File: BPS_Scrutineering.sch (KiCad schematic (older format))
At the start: 26 parts, among them J1 Conn_01x01_Female, J10 Conn_01x01_Female, J11 Conn_01x01_Female, J12 Conn_01x01_Female, J13 Conn_01x01_Female, J14 Conn_01x01_Female, J2 Conn_01x01_Female, J3 Conn_01x01_Female, J4 Conn_01x01_Female, J5 Conn_01x01_Female, J6 Conn_01x01_Female, J7 Conn_01x01_Female, J8 Conn_01x01_Female, J9 Conn_01x01_Female, SW1 SW_DIP_x07, SW2 SW_DIP_x07

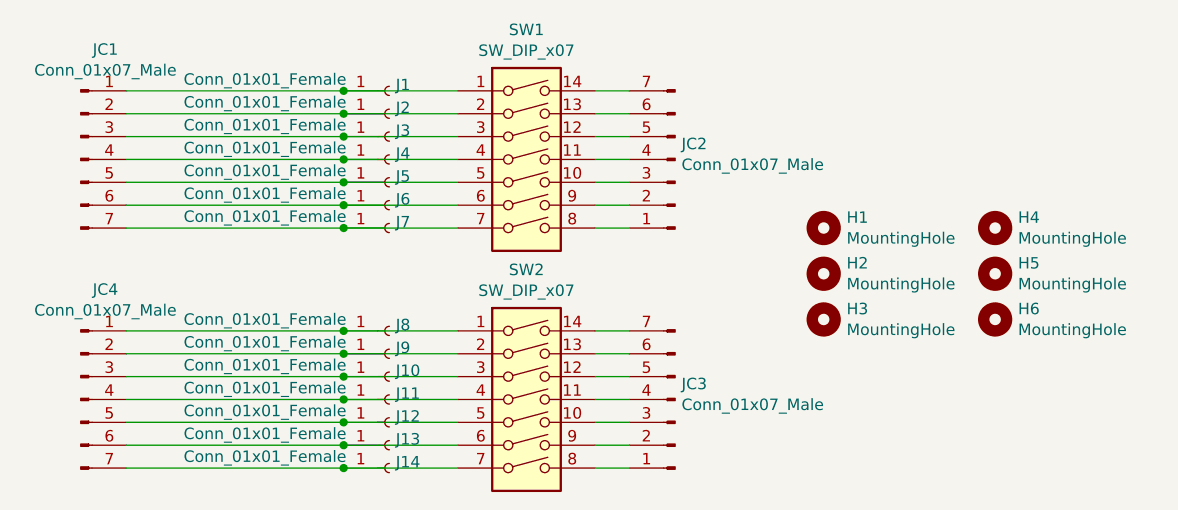
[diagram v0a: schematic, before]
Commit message: Finished PCB
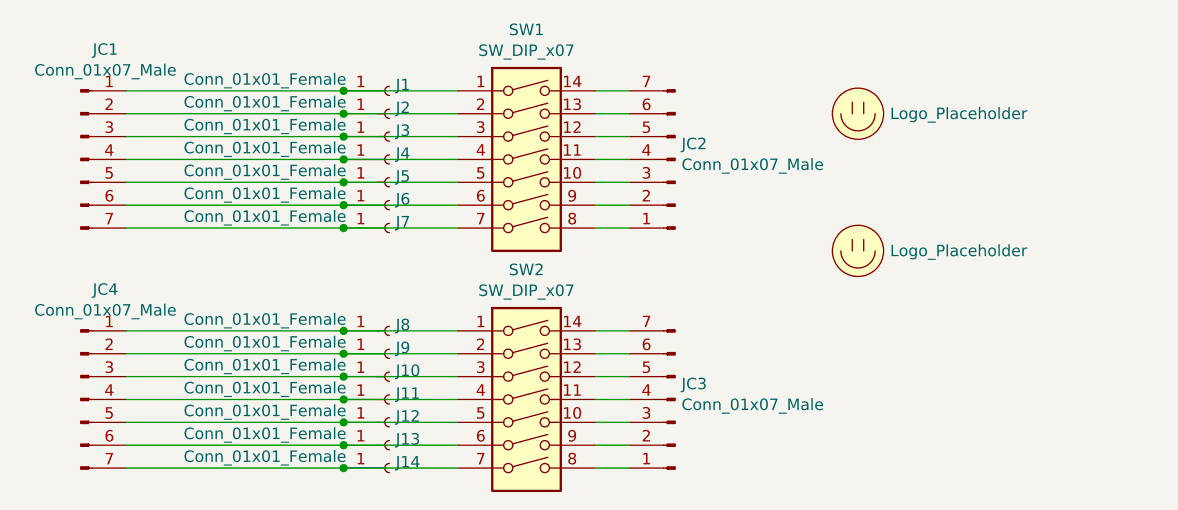
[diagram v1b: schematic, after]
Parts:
- removed H1, H2, H3, H4, H5, H6: MountingHole, MountingHole:MountingHole_3mm, symbol Mechanical:MountingHole
- added LOGO1: Logo_Placeholder, UTSVT_Special:UTSVT_Logo_Symbol, symbol utsvt-misc:Logo_Placeholder
- added LOGO2: Logo_Placeholder, UTSVT_Special:Hallock_Image, symbol utsvt-misc:Logo_Placeholder
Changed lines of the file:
@@
-$EndComp
-$Comp
-L Mechanical:MountingHole H1
-U 1 1 5F9473C1
-P 4650 2000
-F 0 "H1" H 4750 2046 50  0000 L CNN
-F 1 "MountingHole" H 4750 1955 50  0000 L CNN
-F 2 "MountingHole:MountingHole_3mm" H 4650 2000 50  0001 C CNN
-F 3 "~" H 4650 2000 50  0001 C CNN
-	1    4650 2000
-	1    0    0    -1
 $EndComp
 $Comp
@@
 $EndComp
 $Comp
-L Mechanical:MountingHole H2
-U 1 1 5FAEC2DE
-P 4650 2200
-F 0 "H2" H 4750 2246 50  0000 L CNN
-F 1 "MountingHole" H 4750 2155 50  0000 L CNN
-F 2 "MountingHole:MountingHole_3mm" H 4650 2200 50  0001 C CNN
-F 3 "~" H 4650 2200 50  0001 C CNN
-	1    4650 2200
-	1    0    0    -1
-$EndComp
-$Comp
-L Mechanical:MountingHole H3
-U 1 1 5FAF0045
-P 4650 2400
-F 0 "H3" H 4750 2446 50  0000 L CNN
-F 1 "MountingHole" H 4750 2355 50  0000 L CNN
-F 2 "MountingHole:MountingHole_3mm" H 4650 2400 50  0001 C CNN
-F 3 "~" H 4650 2400 50  0001 C CNN
-	1    4650 2400
-	1    0    0    -1
-$EndComp
-$Comp
-L Mechanical:MountingHole H4
-U 1 1 5FAF40EC
-P 5400 2000
-F 0 "H4" H 5500 2046 50  0000 L CNN
-F 1 "MountingHole" H 5500 1955 50  0000 L CNN
-F 2 "MountingHole:MountingHole_3mm" H 5400 2000 50  0001 C CNN
-F 3 "~" H 5400 2000 50  0001 C CNN
-	1    5400 2000
-	1    0    0    -1
-$EndComp
-$Comp
-L Mechanical:MountingHole H5
-U 1 1 5FAF7F09
-P 5400 2200
-F 0 "H5" H 5500 2246 50  0000 L CNN
-F 1 "MountingHole" H 5500 2155 50  0000 L CNN
-F 2 "MountingHole:MountingHole_3mm" H 5400 2200 50  0001 C CNN
-F 3 "~" H 5400 2200 50  0001 C CNN
-	1    5400 2200
-	1    0    0    -1
-$EndComp
-$Comp
-L Mechanical:MountingHole H6
-U 1 1 5FAFBD75
-P 5400 2400
-F 0 "H6" H 5500 2446 50  0000 L CNN
-F 1 "MountingHole" H 5500 2355 50  0000 L CNN
-F 2 "MountingHole:MountingHole_3mm" H 5400 2400 50  0001 C CNN
-F 3 "~" H 5400 2400 50  0001 C CNN
-	1    5400 2400
-	1    0    0    -1
-$EndComp
-$Comp
 L Switch:SW_DIP_x07 SW1
 U 1 1 5FADB5F5
@@
 Wire Wire Line
 	3800 3050 3650 3050
+$Comp
+L utsvt-misc:Logo_Placeholder LOGO1
+U 1 1 5FB02C91
+P 4800 2100
+F 0 "LOGO1" H 4800 2250 50  0001 C CNN
+F 1 "Logo_Placeholder" H 4940 2100 50  0000 L CNN
+F 2 "UTSVT_Special:UTSVT_Logo_Symbol" H 4800 2175 50  0001 C CNN
+F 3 "" H 4800 2175 50  0001 C CNN
+	1    4800 2100
+	1    0    0    -1
+$EndComp
+$Comp
+L utsvt-misc:Logo_Placeholder LOGO2
+U 1 1 5FB04696
+P 4800 1500
+F 0 "LOGO2" H 4800 1650 50  0001 C CNN
+F 1 "Logo_Placeholder" H 4940 1500 50  0000 L CNN
+F 2 "UTSVT_Special:Hallock_Image" H 4800 1575 50  0001 C CNN
+F 3 "" H 4800 1575 50  0001 C CNN
+	1    4800 1500
+	1    0    0    -1
+$EndComp
 $EndSCHEMATC
